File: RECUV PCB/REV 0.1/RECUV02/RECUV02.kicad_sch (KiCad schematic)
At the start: 39 parts, among them P1 VEXT, P2 WJ127-5.0-2P, Q1 MMBT2222ALT1, Q2 MMBT2222ALT1, U1 ESP32-S3-WROOM-1, U2 CH340C, U3 A1117-3.3, U4 RESET, U5 BOOT

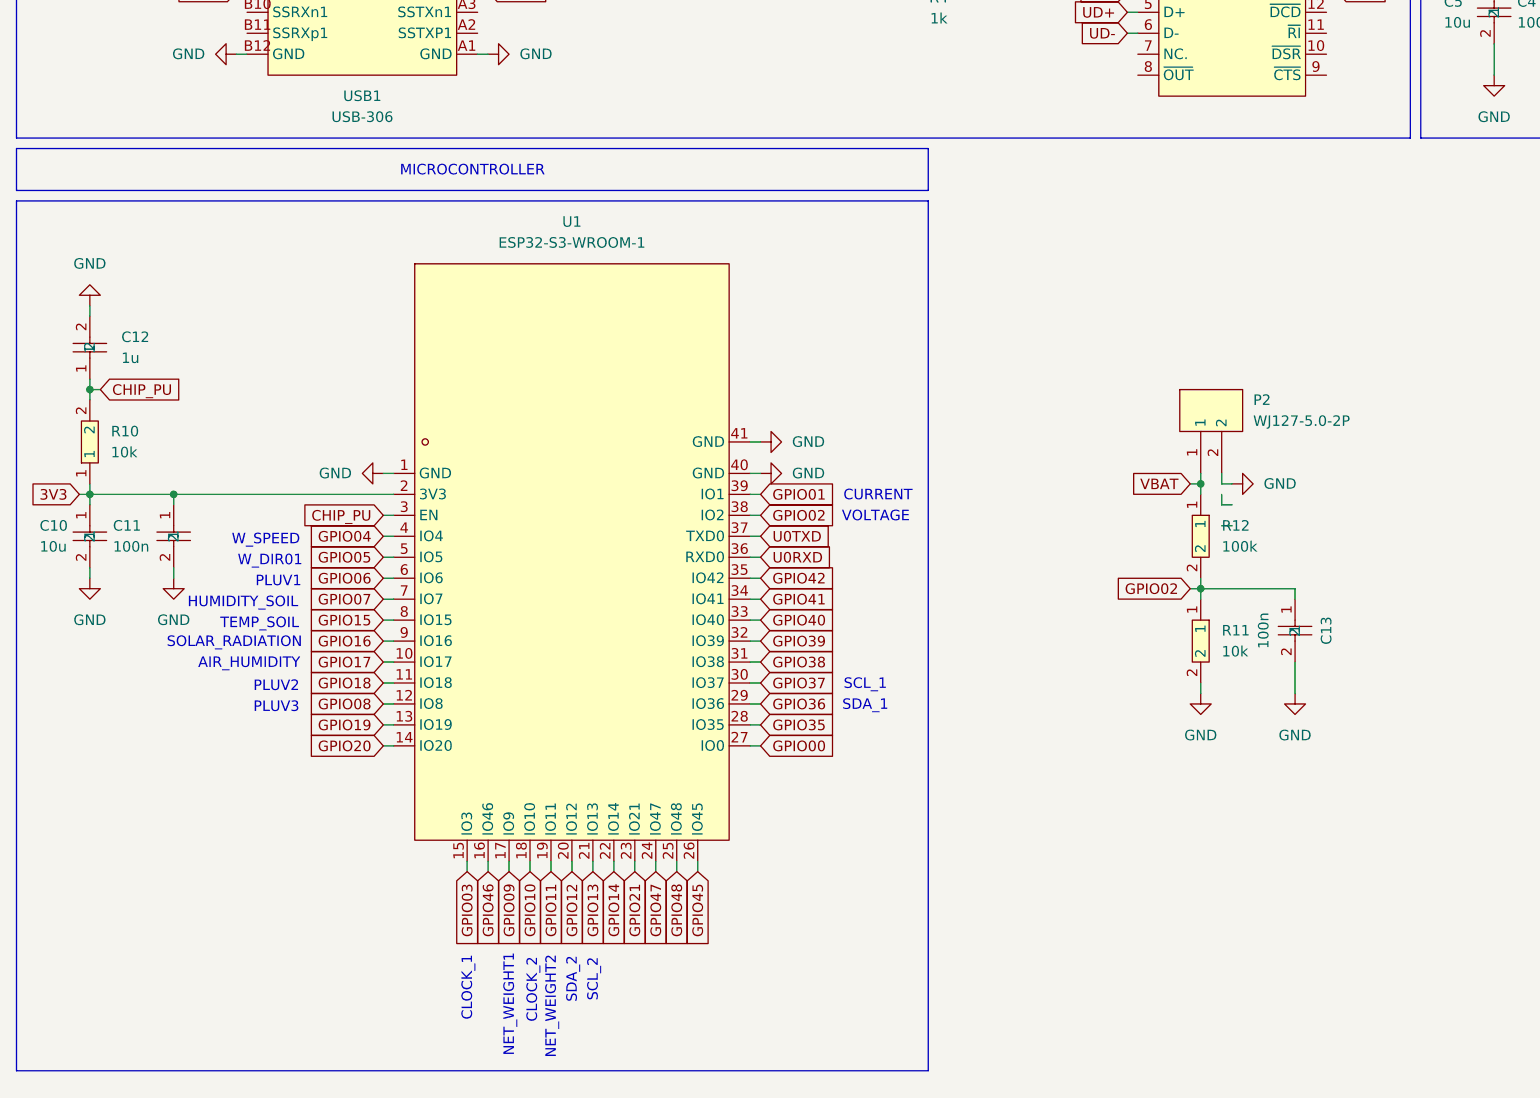
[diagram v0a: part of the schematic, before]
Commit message: Finished electrical sensors
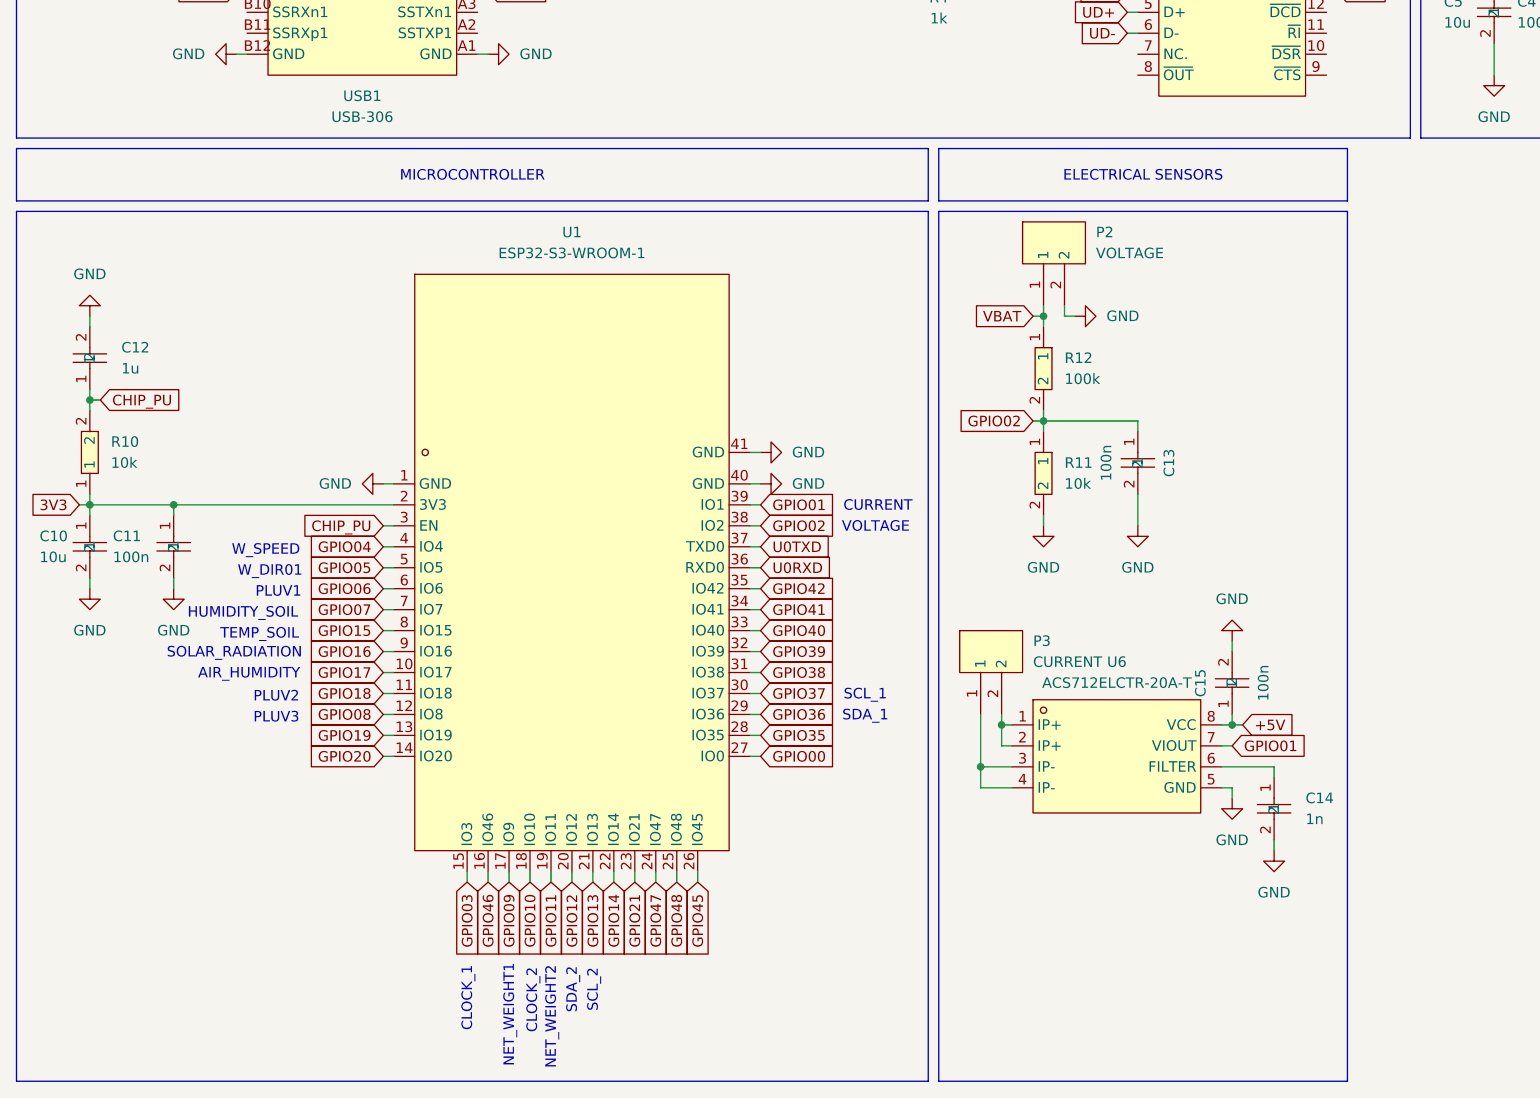
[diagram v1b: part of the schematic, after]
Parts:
- added C14: 1n, EasyEDA:C0805, symbol EasyEDA:CL21C102JBCNNNC
- added C15: 100n, EasyEDA:C0805, symbol EasyEDA:CL21B104KBCNNNC
- added P3: CURRENT, EasyEDA:CONN-TH_2P-P5.00_CPC3703CTR, symbol EasyEDA:WJ127-5.0-2P
- added U6: ACS712ELCTR-20A-T, EasyEDA:SOIC-8_L4.9-W3.9-P1.27-LS6.0-BL, symbol EasyEDA:ACS712ELCTR-20A-T
- P2: value WJ127-5.0-2P -> VOLTAGE
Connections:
- net +5V: now also C15.1, U6.8 (VCC)
- net GND: now also C14.2, C15.2, U6.5 (GND)
- net GPIO01: now also U6.7 (VIOUT)
- new net: P3.2, U6.1 (IP+), U6.2 (IP+)
- new net: P3.1, U6.3 (IP-), U6.4 (IP-)
- new net: C14.1, U6.6 (FILTER)
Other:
- moved on the sheet: C10, C11, C12, C13, P2, R10, R11, R12, U1
